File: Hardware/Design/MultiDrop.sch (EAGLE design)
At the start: 14 parts

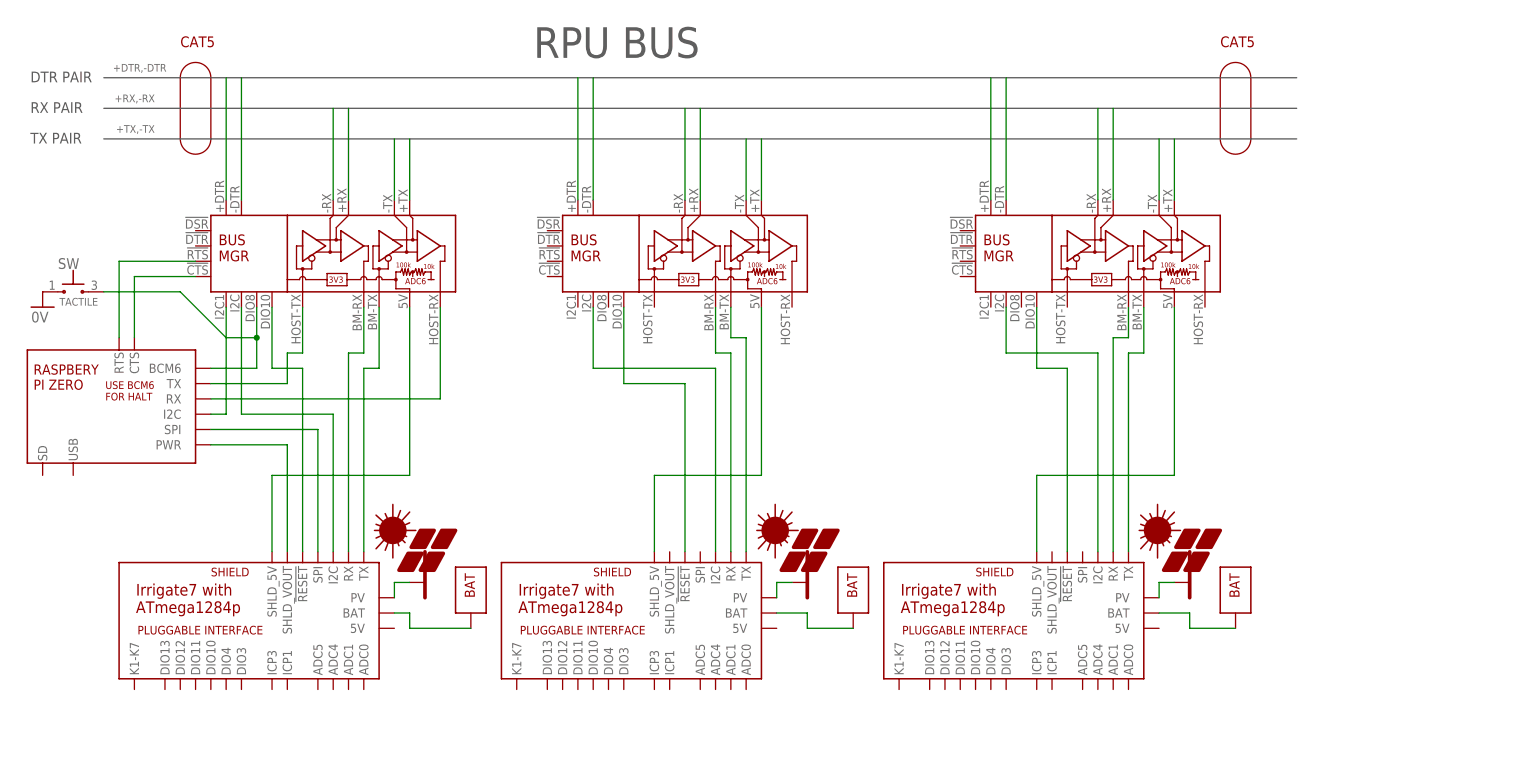
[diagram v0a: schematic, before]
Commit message: Hardware: ^4 schmatic design
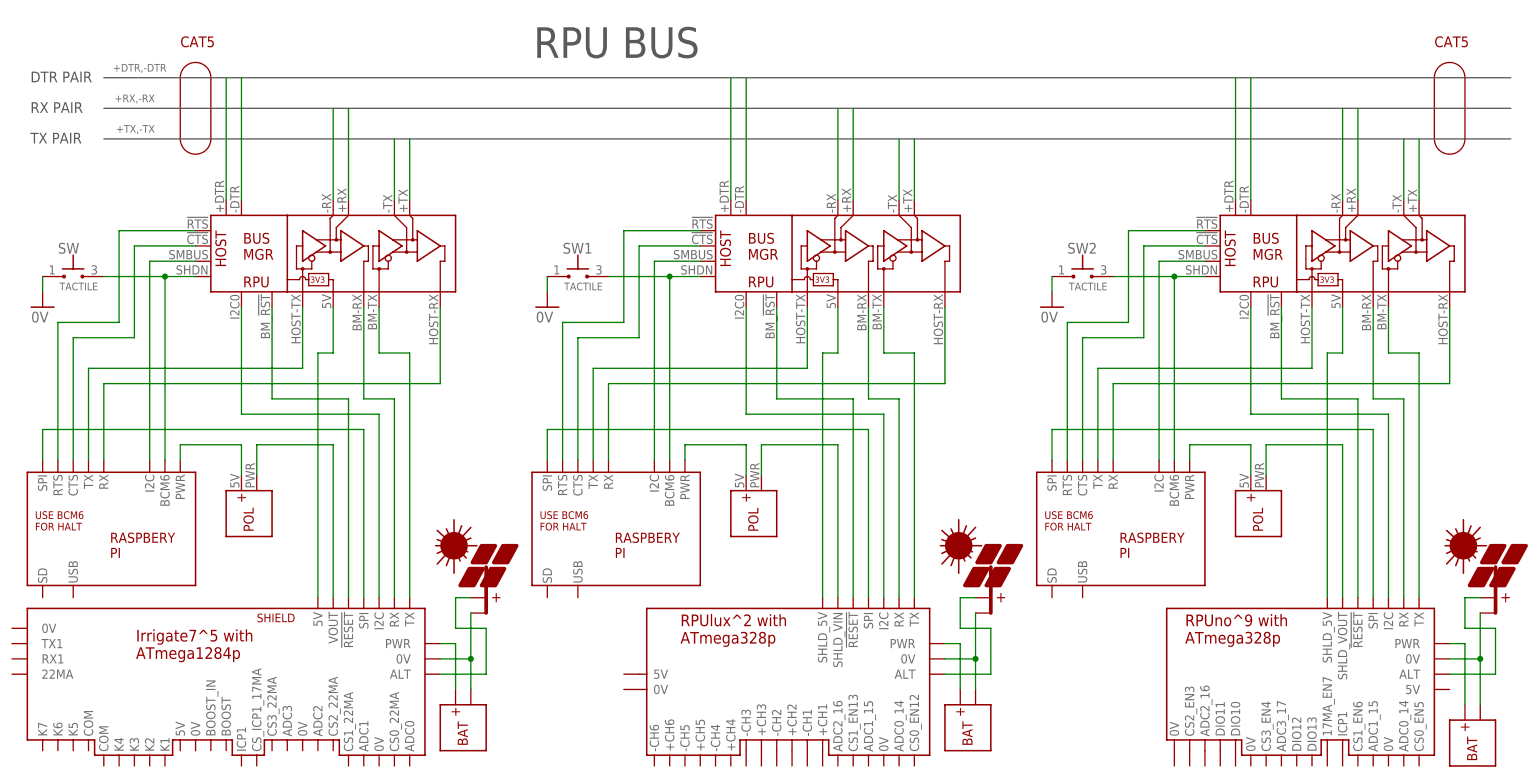
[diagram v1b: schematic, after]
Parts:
- added BM1: (no value), Documentation:RPUNO
- added SW1, SW2: TACTILE, S-Tactile:TAC_SW
- added U$11: PI, Documentation:PI
- added U$12, U$13, U$14: POL, Documentation:POL
- U$1: value BUS_MGR -> IRRIGATE7; device Documentation:BUS_MGR -> Documentation:IRRIGATE7
- U$10, U$5: value BUS_MGR -> PI; device Documentation:BUS_MGR -> Documentation:PI
- U$2: value IRRIGATE7 -> RPULUX; device Documentation:IRRIGATE7 -> Documentation:RPULUX
- U$3: value PI -> BUS_MGR; device Documentation:PI -> Documentation:BUS_MGR
- U$6, U$8: value IRRIGATE7 -> BUS_MGR; device Documentation:IRRIGATE7 -> Documentation:BUS_MGR
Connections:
- removed net +DTR3: U$1.+DTR
- removed net +RX3: U$1.+RX
- removed net +TX3: U$1.+TX
- removed net -DTR3: U$1.-DTR
- removed net -RX3: U$1.-RX
- removed net -TX3: U$1.-TX
- new net +DTR2: U$6.+DTR
- new net +RX2: U$6.+RX
- new net +TX2: U$6.+TX
- new net -DTR2: U$6.-DTR
- new net -RX2: U$6.-RX
- new net -TX2: U$6.-TX
- new net N$16: U$11.RTS, U$8.!RTS
- new net N$18: U$2.SHLD_5V, U$3.PWR
- new net N$19: U$2.!RESET, U$3.BM-!RST!
- new net N$20: U$2.I2C, U$3.I2C0
- new net N$22: U$2.SPI, U$5.SPI
- new net N$23: U$3.SMBUS, U$5.I2C
- new net N$24: SW1.3, U$3.SHDN, U$5.BCM6
- new net N$25: U$3.!CTS, U$5.CTS
- new net N$26: U$3.!RTS, U$5.RTS
- new net N$27: BM1.TX, U$6.BM_TX
- new net N$28: BM1.RX, U$6.BM_RX
- new net N$35: BM1.!RESET, U$6.BM-!RST!
- new net N$37: BM1.SHLD_VOUT, U$14.VIN
- new net N$38: BM1.SPI, U$10.SPI
- new net N$39: U$10.I2C, U$6.SMBUS
- new net N$40: SW2.3, U$10.BCM6, U$6.SHDN
- new net N$42: U$10.RTS, U$6.!RTS
- new net N$46: BM1.0V@2, PV4.-PV, U$7.-BAT
- new net N$47: BM1.PWR, U$7.+BAT
- new net N$49: U$10.PWR, U$14.5V
- new net N$50: U$13.5V, U$5.PWR
- new net N$51: U$11.PWR, U$12.5V
- net +DTR: now also U$8.+DTR; no longer U$10.+DTR
- net +DTR1: now also U$3.+DTR; no longer U$5.+DTR
- net +RX: now also U$8.+RX; no longer U$10.+RX
- net +RX1: now also U$3.+RX; no longer U$5.+RX
- net +TX: now also U$8.+TX; no longer U$10.+TX
- net +TX1: now also U$3.+TX; no longer U$5.+TX
- net -DTR: now also U$8.-DTR; no longer U$10.-DTR
- net -DTR1: now also U$3.-DTR; no longer U$5.-DTR
- net -RX: now also U$8.-RX; no longer U$10.-RX
- net -RX1: now also U$3.-RX; no longer U$5.-RX
- net -TX: now also U$8.-TX; no longer U$10.-TX
- net -TX1: now also U$3.-TX; no longer U$5.-TX
- net 0V: now also SW1.1, SW2.1
- net N$1: now also U$1.TX, U$8.BM_TX; no longer U$10.BM_TX, U$8.TX
- net N$10: now also U$2.TX, U$3.BM_TX; no longer U$5.BM_TX, U$6.TX
- net N$11: now also U$2.RX, U$3.BM_RX; no longer U$5.BM_RX, U$6.RX
- net N$12: now also U$1.PWR, U$4.+BAT; no longer U$4.BAT_PWR, U$8.BAT
- net N$13: now also U$11.CTS, U$8.!CTS; no longer SW.3, U$10.DIO8, U$3.BCM6
- net N$14: now also U$3.HOST_RX, U$5.RX; no longer U$1.BM_TX, U$2.TX
- net N$15: now also PV1.+PV, U$1.ALT; no longer U$10.I2C1, U$3.I2C
- net N$17: now also U$3.HOST_TX, U$5.TX; no longer U$6.BAT, U$9.BAT_PWR
- net N$2: now also U$1.RX, U$8.BM_RX; no longer U$10.BM_RX, U$8.RX
- net N$21: now also U$13.VIN, U$2.SHLD_VIN; no longer U$1.BM_RX, U$2.RX
- net N$29: now also U$1.5V@SHLD, U$8.PWR; no longer U$10.PWR, U$8.SHLD_5V
- net N$3: now also U$1.VOUT, U$12.VIN; no longer U$3.PWR, U$8.SHLD_VOUT
- net N$30: now also U$1.!RESET, U$8.BM-!RST!; no longer U$10.DIO10, U$8.!RESET
- net N$31: now also U$10.RX, U$6.HOST_RX; no longer U$2.BAT, U$7.BAT_PWR
- net N$32: now also U$10.TX, U$6.HOST_TX; no longer U$1.I2C, U$2.I2C
- net N$33: now also U$1.I2C, U$8.I2C0; no longer U$10.I2C, U$8.I2C
- net N$34: now also BM1.SHLD_5V, U$6.PWR; no longer PV4.PV_PWR, U$2.PV
- net N$36: now also BM1.I2C, U$6.I2C0; no longer PV2.PV_PWR, U$6.PV
- net N$4: now also U$11.I2C, U$8.SMBUS; no longer U$10.!CTS, U$3.CTS
- net N$41: now also U$10.CTS, U$6.!CTS; no longer U$1.PWR, U$2.SHLD_5V
- net N$43: now also PV2.-PV, U$2.0V@2, U$9.-BAT; no longer U$1.DIO10, U$2.!RESET
- net N$44: now also U$2.PWR, U$9.+BAT; no longer U$5.DIO10, U$6.!RESET
- net N$45: now also PV2.+PV, U$2.ALT; no longer U$5.PWR, U$6.SHLD_5V
- net N$48: now also BM1.ALT, PV4.+PV; no longer U$5.I2C, U$6.I2C
- net N$5: now also SW.3, U$11.BCM6, U$8.SHDN; no longer U$10.!RTS, U$3.RTS
- net N$6: now also U$1.SPI, U$11.SPI; no longer U$3.SPI, U$8.SPI
- net N$7: now also PV1.-PV, U$1.0V@PWR, U$4.-BAT; no longer PV1.PV_PWR, U$8.PV
- net N$8: now also U$11.RX, U$8.HOST_RX; no longer U$10.HOST_RX, U$3.RX
- net N$9: now also U$11.TX, U$8.HOST_TX; no longer U$10.HOST_TX, U$3.TX
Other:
- note removed: "3W PV"
- note removed: "7.5AHr"
- note removed: "RPUadpt"
- note removed: "USB WiFi USB Ethernet USB OTG"
- moved on the sheet: SW
